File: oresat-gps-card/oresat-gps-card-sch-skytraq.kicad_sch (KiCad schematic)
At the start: 8 parts, among them U23 ORION-B16

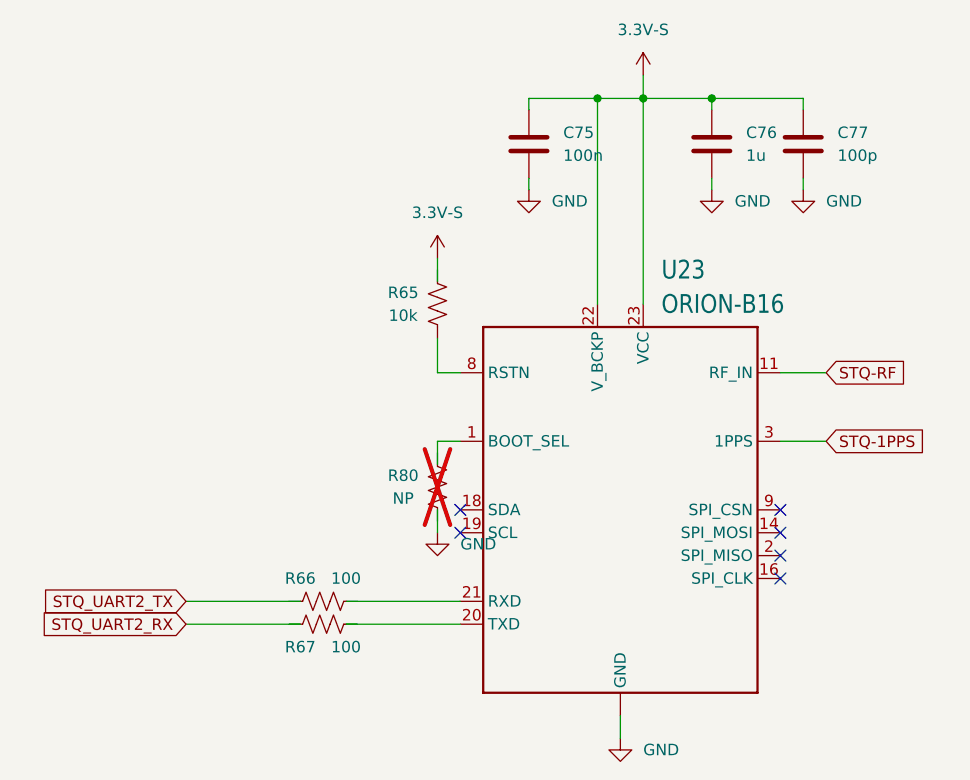
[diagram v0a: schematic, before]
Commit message: Routine Push
First attempt to clean up schematic
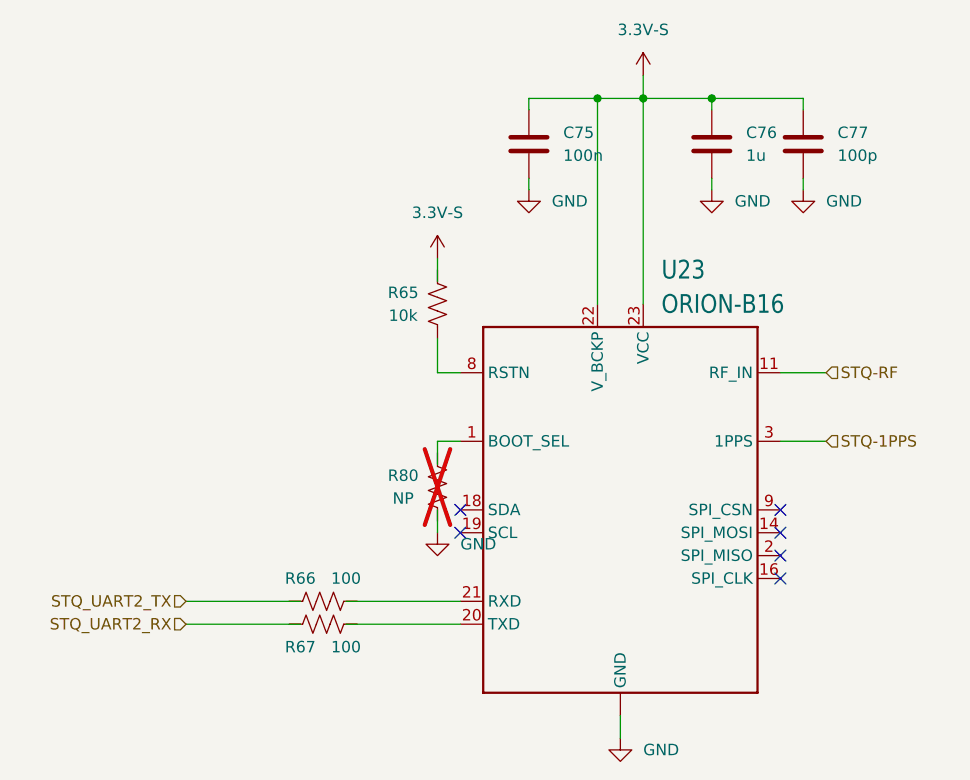
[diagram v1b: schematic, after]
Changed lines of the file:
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@@
 		)
 	)
-	(global_label "STQ_UART2_RX"
+	(hierarchical_label "STQ-RF"
+		(shape input)
+		(at 238.76 119.38 0)
+		(effects
+			(font
+				(size 1.27 1.27)
+			)
+			(justify left)
+		)
+	)
+	(hierarchical_label "STQ-1PPS"
+		(shape input)
+		(at 238.76 127 0)
+		(effects
+			(font
+				(size 1.27 1.27)
+			)
+			(justify left)
+		)
+	)
+	(hierarchical_label "STQ_UART2_RX"
 		(shape input)
 		(at 167.64 147.32 180)
-		(fields_autoplaced yes)
 		(effects
 			(font
@@
 			(justify right)
 		)
-		(property "Intersheetrefs" "${INTERSHEET_REFS}"
-			(at 151.4383 147.2406 0)
-			(show_name no)
-			(do_not_autoplace no)
-			(effects
-				(font
-					(size 1.27 1.27)
-				)
-				(justify right)
-			)
-		)
 	)
-	(global_label "STQ-1PPS"
-		(shape input)
-		(at 238.76 127 0)
-		(fields_autoplaced yes)
-		(effects
-			(font
-				(size 1.27 1.27)
-			)
-			(justify left)
-		)
-		(property "Intersheetrefs" "${INTERSHEET_REFS}"
-			(at 251.2121 126.9206 0)
-			(show_name no)
-			(do_not_autoplace no)
-			(effects
-				(font
-					(size 1.27 1.27)
-				)
-				(justify left)
-			)
-		)
-	)
-	(global_label "STQ-RF"
-		(shape input)
-		(at 238.76 119.38 0)
-		(fields_autoplaced yes)
-		(effects
-			(font
-				(size 1.27 1.27)
-			)
-			(justify left)
-		)
-		(property "Intersheetrefs" "${INTERSHEET_REFS}"
-			(at 248.6117 119.3006 0)
-			(show_name no)
-			(do_not_autoplace no)
-			(effects
-				(font
-					(size 1.27 1.27)
-				)
-				(justify left)
-			)
-		)
-	)
-	(global_label "STQ_UART2_TX"
+	(hierarchical_label "STQ_UART2_TX"
 		(shape input)
 		(at 167.64 144.78 180)
-		(fields_autoplaced yes)
 		(effects
 			(font
@@
 			(justify right)
 		)
-		(property "Intersheetrefs" "${INTERSHEET_REFS}"
-			(at 151.7407 144.7006 0)
-			(show_name no)
-			(do_not_autoplace no)
-			(effects
-				(font
-					(size 1.27 1.27)
-				)
-				(justify right)
-			)
-		)
 	)

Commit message: Routine Push
Schematic finished. Components laid out, chasing ERCs.
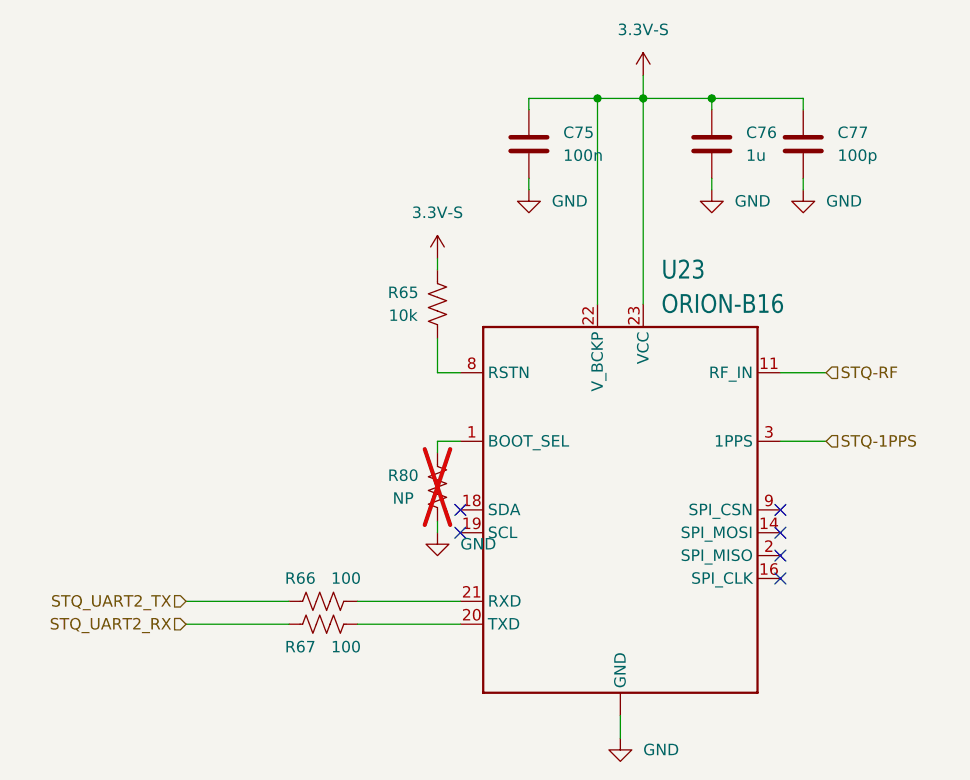
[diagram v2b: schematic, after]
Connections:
- net 3.3V-S: now also R65.1
- net GND: now also R80.2
- net STQ_UART2_RX: now also R67.1
- net STQ_UART2_TX: now also R66.1
- net at R67.2: now also U23.20 (TXD)
- net at U23.1 (BOOT_SEL): now also R80.1
- net at U23.21 (RXD): now also R66.2
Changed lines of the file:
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@@
+	(wire
+		(pts
+			(xy 195.58 106.68) (xy 195.58 107.95)
+		)
+		(stroke
+			(width 0)
+			(type default)
+		)
+	)
 	(wire
 		(pts
@@
 	(wire
 		(pts
+			(xy 167.64 147.32) (xy 179.07 147.32)
+		)
+		(stroke
+			(width 0)
+			(type default)
+		)
+	)
+	(wire
+		(pts
 			(xy 213.36 88.9) (xy 218.44 88.9)
 		)
@@
 	(wire
 		(pts
-			(xy 195.58 127) (xy 195.58 129.54)
-		)
-		(stroke
-			(width 0)
-			(type default)
-		)
-	)
-	(wire
-		(pts
-			(xy 195.58 106.68) (xy 195.58 109.22)
+			(xy 186.69 147.32) (xy 198.12 147.32)
 		)
 		(stroke
@@
 	(wire
 		(pts
-			(xy 167.64 147.32) (xy 180.34 147.32)
-		)
-		(stroke
-			(width 0)
-			(type default)
-		)
-	)
-	(wire
-		(pts
 			(xy 213.36 111.76) (xy 213.36 88.9)
 		)
@@
 	(wire
 		(pts
-			(xy 195.58 134.62) (xy 195.58 137.16)
+			(xy 186.69 144.78) (xy 198.12 144.78)
+		)
+		(stroke
+			(width 0)
+			(type default)
+		)
+	)
+	(wire
+		(pts
+			(xy 167.64 144.78) (xy 179.07 144.78)
 		)
 		(stroke
@@
 	(wire
 		(pts
+			(xy 195.58 135.89) (xy 195.58 137.16)
+		)
+		(stroke
+			(width 0)
+			(type default)
+		)
+	)
+	(wire
+		(pts
+			(xy 195.58 127) (xy 195.58 128.27)
+		)
+		(stroke
+			(width 0)
+			(type default)
+		)
+	)
+	(wire
+		(pts
 			(xy 233.68 127) (xy 238.76 127)
 		)
@@
 	(wire
 		(pts
-			(xy 185.42 147.32) (xy 198.12 147.32)
-		)
-		(stroke
-			(width 0)
-			(type default)
-		)
-	)
-	(wire
-		(pts
 			(xy 205.74 88.9) (xy 205.74 90.17)
 		)
 		(stroke
-			(width 0)
-			(type default)
-		)
-	)
-	(wire
-		(pts
-			(xy 185.42 144.78) (xy 198.12 144.78)
-		)
-		(stroke
-			(width 0)
-			(type default)
-		)
-	)
-	(wire
-		(pts
-			(xy 167.64 144.78) (xy 180.34 144.78)
-		)
-		(stroke
